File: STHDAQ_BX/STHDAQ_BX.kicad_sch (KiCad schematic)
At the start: 48 parts, among them J1 532611071, P1 S2B-PH-SM4-TB, U1 ADS1256IDBR, U2 ADP151AUJZ-3.0-R7, U3 OPA350UA, U4 REF5025AIDR, U5 102010448, U6 LT1461AIS8-5-PBF, Y1 ABLS-8MHZ-K4T

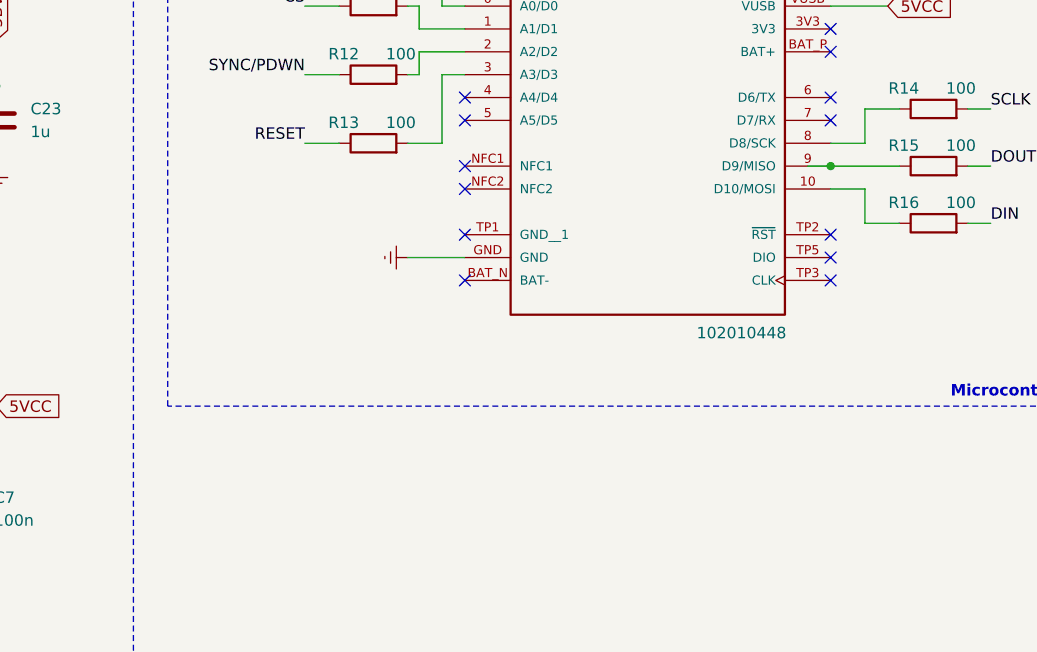
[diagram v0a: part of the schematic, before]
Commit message: BX pcb layouting
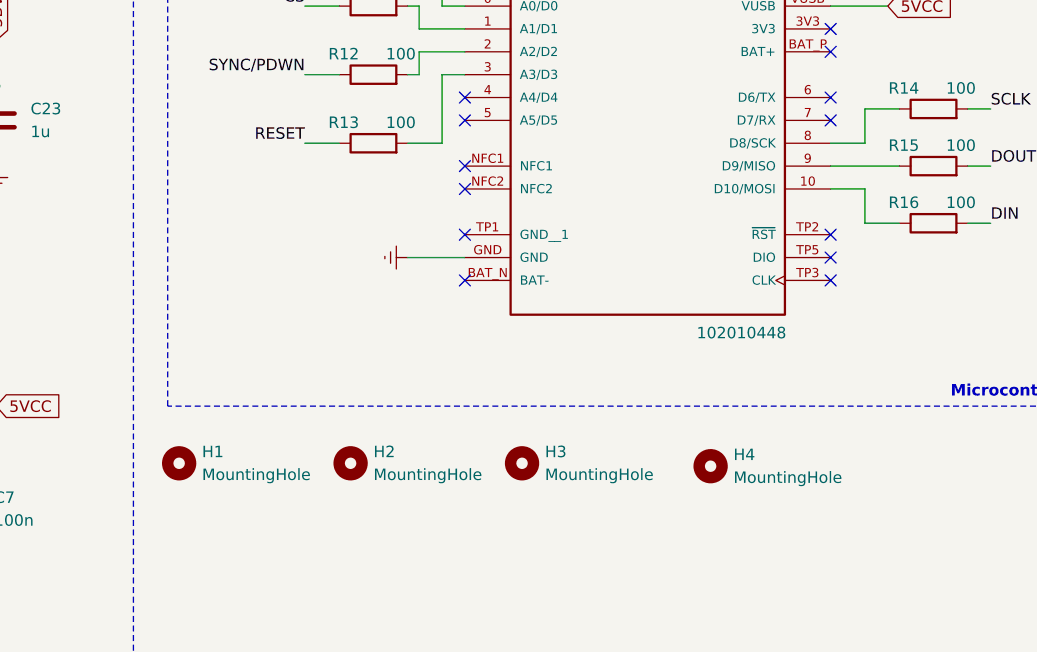
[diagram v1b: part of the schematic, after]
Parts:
- added H1, H2, H3, H4: MountingHole, MountingHole:MountingHole_3.2mm_M3_ISO14580_Pad_TopBottom, symbol Mechanical:MountingHole
- P1: footprint daFootprints:JST_S2B-PH-SM4-TB -> daFootprintsBX:JST_S2B-PH-SM4-TB
- U6: footprint daFootprints:SOIC127P600X175-8N -> daFootprintsBX:SOIC127P600X175-8N
